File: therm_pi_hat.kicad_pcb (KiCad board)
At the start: 2 copper layers, 65 x 56.5 mm, 50 parts, among them J1 1935161, J2 LCD Header, J3 Raspberry_Pi_2_3, J4 SJ1-3533NG, J5 SJ1-3533NG, J6 SJ1-3533NG, J7 SJ1-3533NG, Q1 Q_NPN_BCE, SW1 D6C10 F1 LFS, SW2 D6C10 F1 LFS, SW3 D6C10 F1 LFS, SW4 D6C10 F1 LFS, U1 ADS1118IDGS, U2 ADS1118IDGS

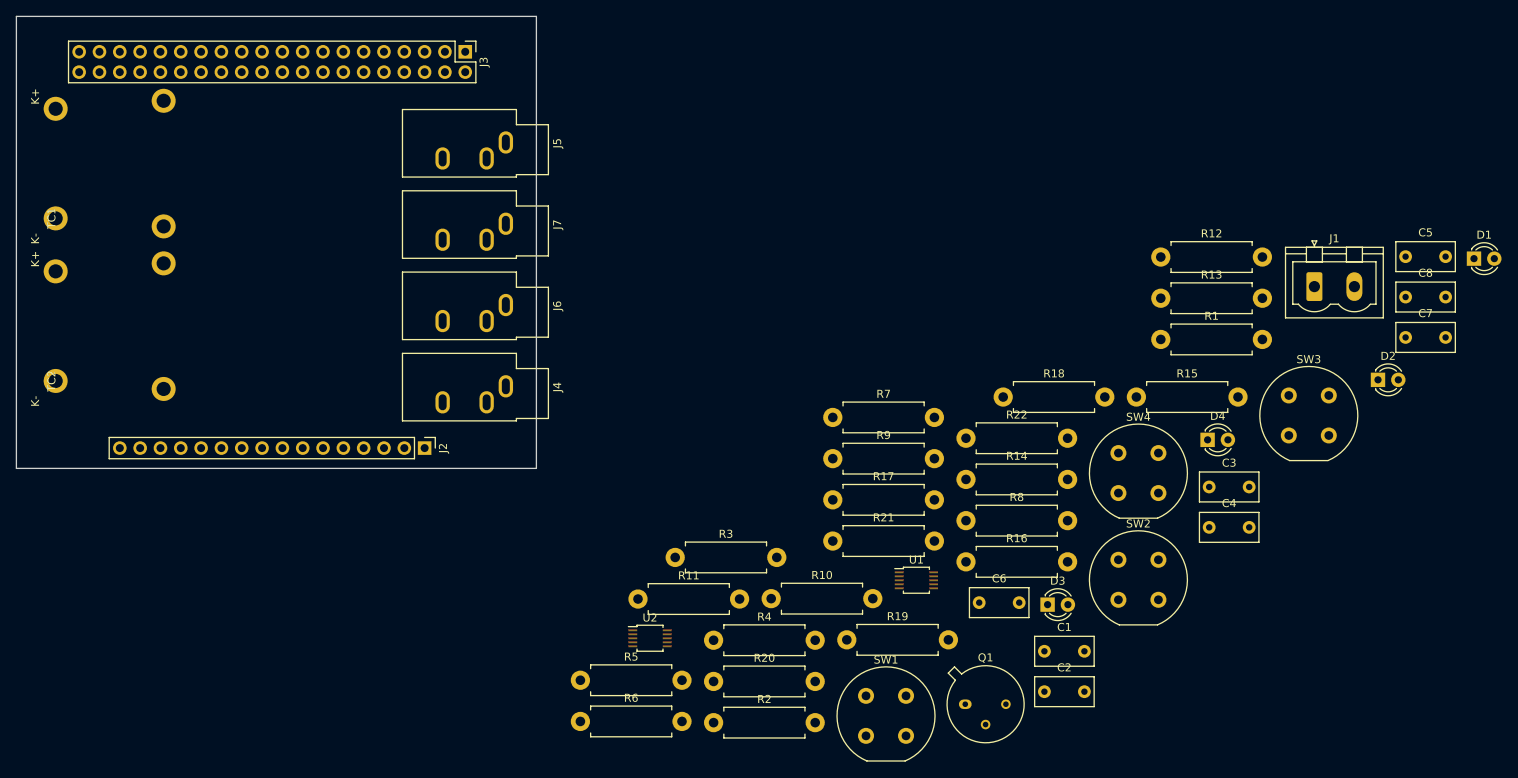
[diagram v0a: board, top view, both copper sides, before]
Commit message: continued placement
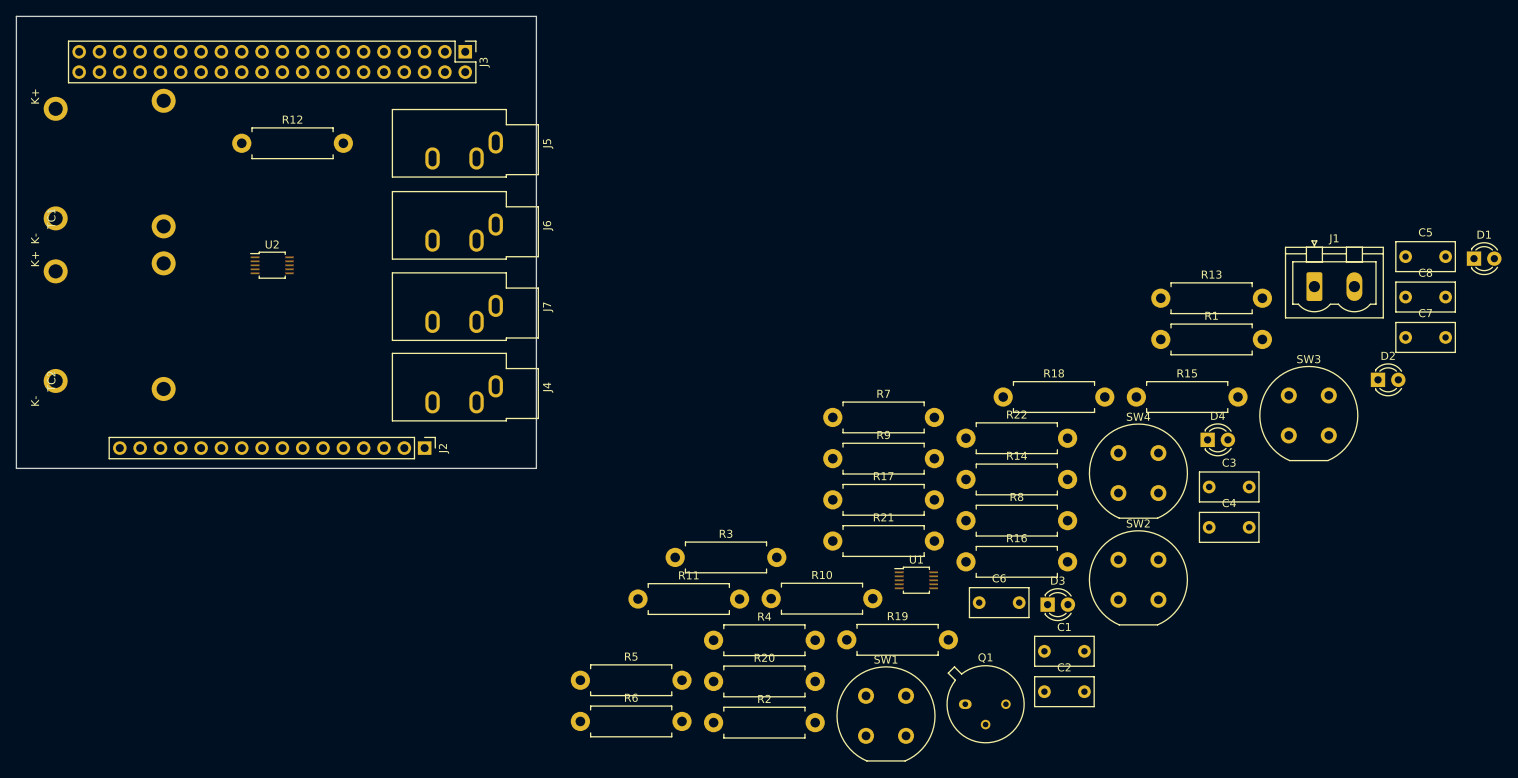
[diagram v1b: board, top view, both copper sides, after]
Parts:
- moved R12 115.8 mm to (54.6, 55.9)
- moved U2 66.4 mm to (58.4, 71.1)
- moved J7 10.3 mm to (86.4, 76.2)
- moved J6 10.1 mm to (86.4, 66.0)
- moved J4 1.26 mm to (86.4, 86.3)
- moved J5 1.26 mm to (86.4, 55.8)
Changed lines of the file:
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@@
   )
   (footprint "Package_SO:TSSOP-10_3x3mm_P0.5mm" (layer "F.Cu")
-    (at 105.64 117.75)
+    (at 58.42 71.12)
     (descr "TSSOP10: plastic thin shrink small outline package; 10 leads; body width 3 mm; (see NXP SSOP-TSSOP-VSO-REFLOW.pdf and sot552-1_po.pdf)")
     (tags "SSOP 0.5")
@@
   )
   (footprint "Connector_Audio:Jack_3.5mm_CUI_SJ1-3533NG_Horizontal" (layer "F.Cu")
-    (at 87.62 65.94 -90)
+    (at 86.36 76.2 -90)
     (descr "TRS 3.5mm, horizontal, through-hole, https://www.cui.com/product/resource/sj1-353xng.pdf")
     (tags "TRS audio jack stereo horizontal")
@@
   )
   (footprint "Connector_Audio:Jack_3.5mm_CUI_SJ1-3533NG_Horizontal" (layer "F.Cu")
-    (at 87.62 55.78 -90)
+    (at 86.36 55.78 -90)
     (descr "TRS 3.5mm, horizontal, through-hole, https://www.cui.com/product/resource/sj1-353xng.pdf")
     (tags "TRS audio jack stereo horizontal")
@@
   )
   (footprint "Connector_Audio:Jack_3.5mm_CUI_SJ1-3533NG_Horizontal" (layer "F.Cu")
-    (at 87.62 76.1 -90)
+    (at 86.36 66.04 -90)
     (descr "TRS 3.5mm, horizontal, through-hole, https://www.cui.com/product/resource/sj1-353xng.pdf")
     (tags "TRS audio jack stereo horizontal")
@@
   )
   (footprint "Resistor_THT:R_Axial_DIN0411_L9.9mm_D3.6mm_P12.70mm_Horizontal" (layer "F.Cu")
-    (at 169.49 70.1)
+    (at 54.61 55.88)
     (descr "Resistor, Axial_DIN0411 series, Axial, Horizontal, pin pitch=12.7mm, 1W, length*diameter=9.9*3.6mm^2")
     (tags "Resistor Axial_DIN0411 series Axial Horizontal pin pitch 12.7mm 1W length 9.9mm diameter 3.6mm")
@@
   )
   (footprint "Connector_Audio:Jack_3.5mm_CUI_SJ1-3533NG_Horizontal" (layer "F.Cu")
-    (at 87.62 86.26 -90)
+    (at 86.36 86.26 -90)
     (descr "TRS 3.5mm, horizontal, through-hole, https://www.cui.com/product/resource/sj1-353xng.pdf")
     (tags "TRS audio jack stereo horizontal")
